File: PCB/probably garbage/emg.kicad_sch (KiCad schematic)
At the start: 102 parts, among them J1 USB_C_Receptacle_USB2.0_16P, J2 BAT+, J3 BAT-, SW1 RotaryEncoder_Switch_MP, SW10 2,2, SW11 2,3, SW12 2,4, SW13 2,5, SW14 3,1, SW15 3,2, SW16 3,3, SW17 3,4, SW18 3,5, SW19 4,1, SW2 EN, SW20 4,2, SW21 4,3, SW22 4,4, SW23 4,5, SW24 5,1, SW25 5,2, SW26 5,3, SW27 5,4, SW28 5,5, SW29 6,1, SW3 BOOT, SW30 6,2, SW31 6,3, SW32 6,4, SW33 6,5, SW34 7,1, SW35 7,2, SW36 7,3, SW37 7,4, SW38 7,5, SW4 1,1, SW5 1,2, SW6 1,3, SW7 1,4, SW8 1,5, SW9 2,1, U1 NCP1117-3.3_SOT223, U2 TVS1400DRV, U3 NCP1117-3.3_SOT223, U4 USBLC6-2SC6, U5 ESP32-C6-MINI-1

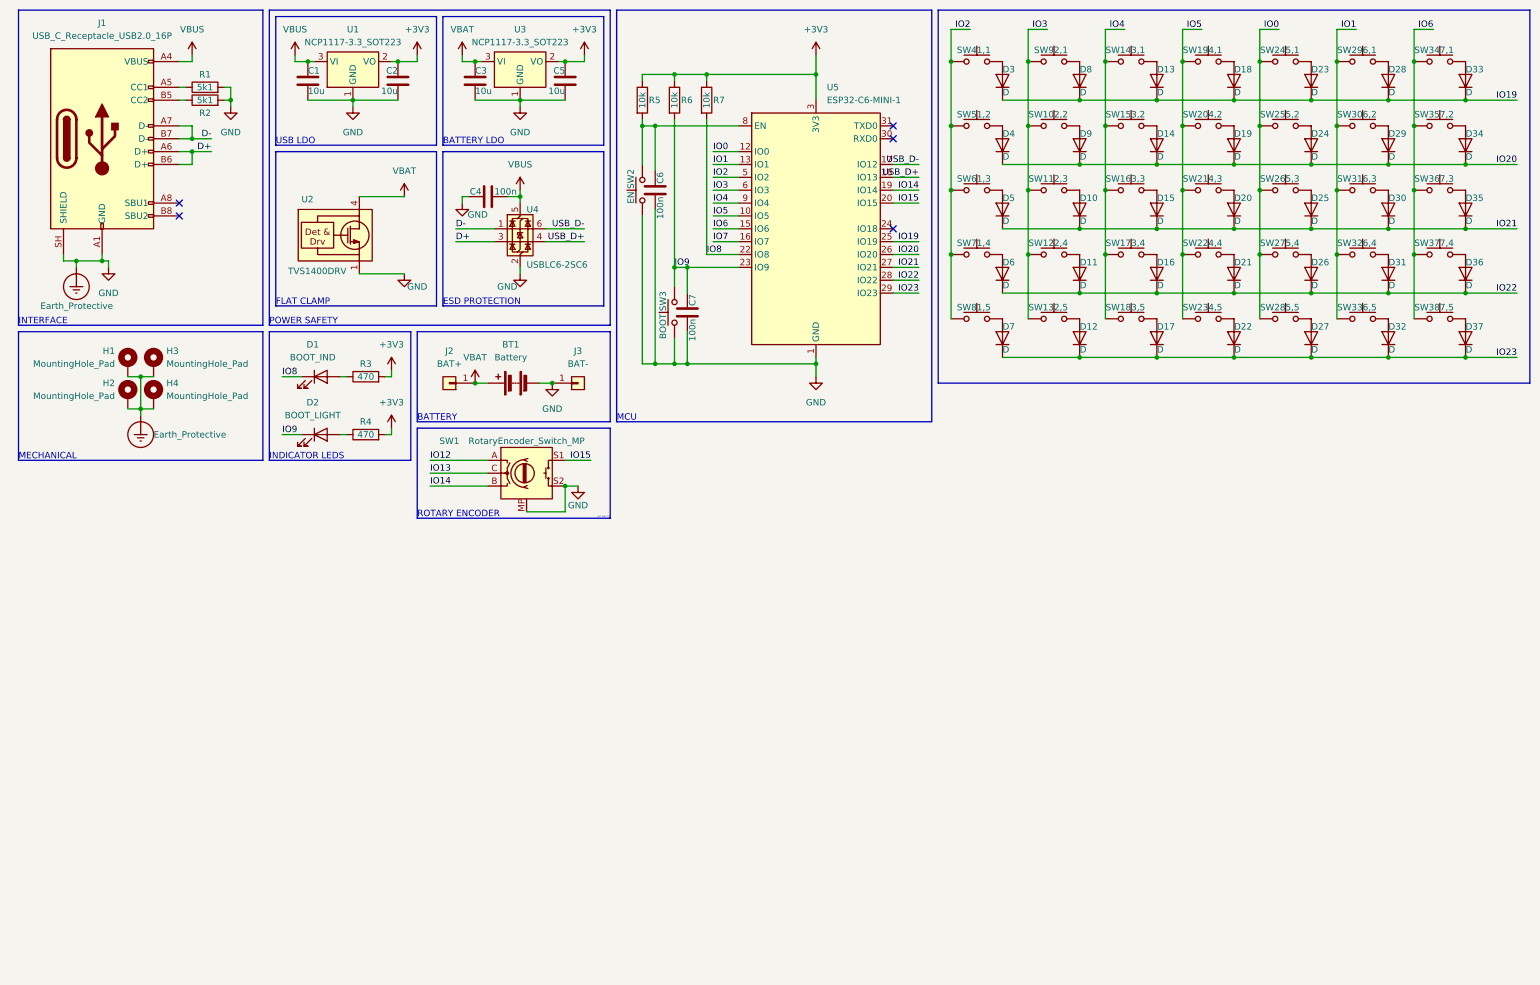
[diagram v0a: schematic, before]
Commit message: file organization
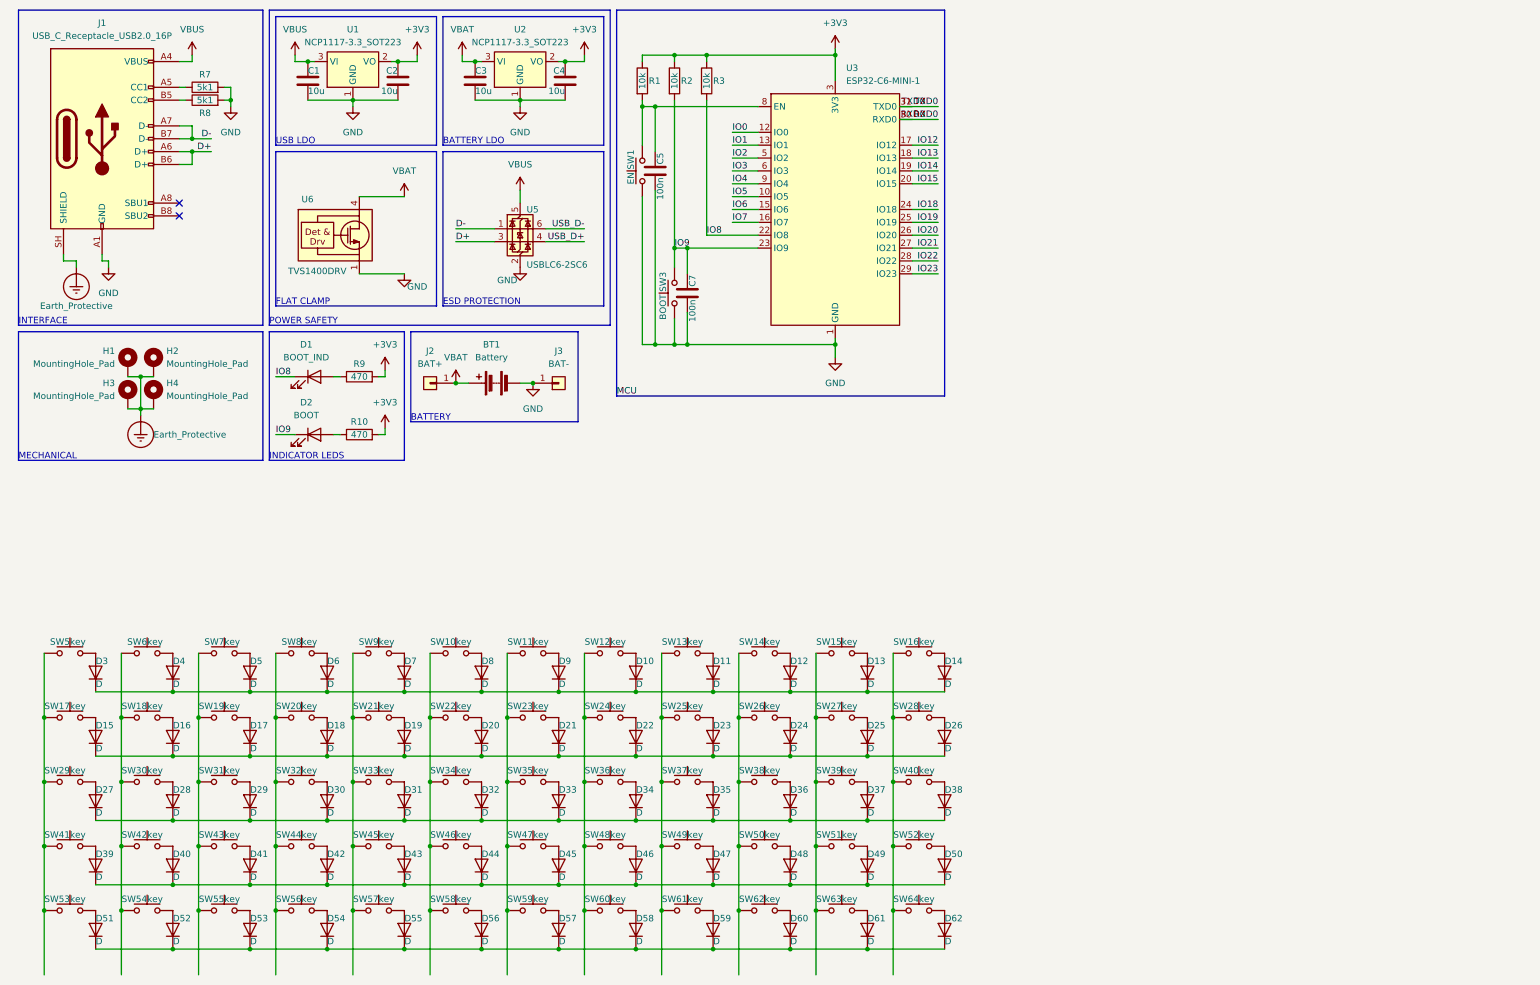
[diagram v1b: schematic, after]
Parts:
- removed C4: 100n, Diode_SMD:D_0805_2012Metric, symbol Device:C
- removed SW1: RotaryEncoder_Switch_MP, Rotary_Encoder:RotaryEncoder_Alps_EC12E-Switch_Vertical_H20mm_CircularMountingHoles, symbol Device:RotaryEncoder_Switch_MP
- added D10, D11, D12, D13, D14, D22, D23, D24, D25, D26, D34, D35, D36, D37, D38, D46, D47, D48, D49, D50, D58, D59, D60, D61, D62: D, symbol Device:D
- added SW12, SW13, SW14, SW15, SW16, SW24, SW25, SW26, SW27, SW28, SW36, SW37, SW38, SW39, SW40, SW48, SW49, SW50, SW51, SW52, SW60, SW61, SW62, SW63, SW64: key, symbol Switch:SW_Push
- BT1: footprint Battery:BatteryHolder_Keystone_1042_1x18650 -> (none)
- C1, C2, C3, C7, D1, D3: footprint Diode_SMD:D_0805_2012Metric -> (none)
- C4: renamed from C5; footprint Diode_SMD:D_0805_2012Metric -> (none)
- C5: renamed from C6; footprint Diode_SMD:D_0805_2012Metric -> (none)
- D15: renamed from D4; footprint Diode_SMD:D_0805_2012Metric -> (none)
- D16: renamed from D9; footprint Diode_SMD:D_0805_2012Metric -> (none)
- D17: renamed from D14; footprint Diode_SMD:D_0805_2012Metric -> (none)
- D18: renamed from D19; footprint Diode_SMD:D_0805_2012Metric -> (none)
- D19: renamed from D24; footprint Diode_SMD:D_0805_2012Metric -> (none)
- D2: value BOOT_LIGHT -> BOOT; footprint Diode_SMD:D_0805_2012Metric -> (none)
- D20: renamed from D29; footprint Diode_SMD:D_0805_2012Metric -> (none)
- D21: renamed from D34; footprint Diode_SMD:D_0805_2012Metric -> (none)
- D27: renamed from D5; footprint Diode_SMD:D_0805_2012Metric -> (none)
- D28: renamed from D10; footprint Diode_SMD:D_0805_2012Metric -> (none)
- D29: renamed from D15; footprint Diode_SMD:D_0805_2012Metric -> (none)
- D30: renamed from D20; footprint Diode_SMD:D_0805_2012Metric -> (none)
- D31: renamed from D25; footprint Diode_SMD:D_0805_2012Metric -> (none)
- D32: renamed from D30; footprint Diode_SMD:D_0805_2012Metric -> (none)
- D33: renamed from D35; footprint Diode_SMD:D_0805_2012Metric -> (none)
- D39: renamed from D6; footprint Diode_SMD:D_0805_2012Metric -> (none)
- D4: renamed from D8; footprint Diode_SMD:D_0805_2012Metric -> (none)
- D40: renamed from D11; footprint Diode_SMD:D_0805_2012Metric -> (none)
- D41: renamed from D16; footprint Diode_SMD:D_0805_2012Metric -> (none)
- D42: renamed from D21; footprint Diode_SMD:D_0805_2012Metric -> (none)
- D43: renamed from D26; footprint Diode_SMD:D_0805_2012Metric -> (none)
- D44: renamed from D31; footprint Diode_SMD:D_0805_2012Metric -> (none)
- D45: renamed from D36; footprint Diode_SMD:D_0805_2012Metric -> (none)
- D5: renamed from D13; footprint Diode_SMD:D_0805_2012Metric -> (none)
- D51: renamed from D7; footprint Diode_SMD:D_0805_2012Metric -> (none)
- D52: renamed from D12; footprint Diode_SMD:D_0805_2012Metric -> (none)
- D53: renamed from D17; footprint Diode_SMD:D_0805_2012Metric -> (none)
- D54: renamed from D22; footprint Diode_SMD:D_0805_2012Metric -> (none)
- D55: renamed from D27; footprint Diode_SMD:D_0805_2012Metric -> (none)
- D56: renamed from D32; footprint Diode_SMD:D_0805_2012Metric -> (none)
- D57: renamed from D37; footprint Diode_SMD:D_0805_2012Metric -> (none)
- D6: renamed from D18; footprint Diode_SMD:D_0805_2012Metric -> (none)
- D7: renamed from D23; footprint Diode_SMD:D_0805_2012Metric -> (none)
- D8: renamed from D28; footprint Diode_SMD:D_0805_2012Metric -> (none)
- D9: renamed from D33; footprint Diode_SMD:D_0805_2012Metric -> (none)
- H1, H4: footprint MountingHole:MountingHole_3.2mm_M3_Pad -> (none)
- H2: renamed from H3; footprint MountingHole:MountingHole_3.2mm_M3_Pad -> (none)
- H3: renamed from H2; footprint MountingHole:MountingHole_3.2mm_M3_Pad -> (none)
- J1: footprint Connector_USB:USB_C_Receptacle_GCT_USB4105-xx-A_16P_TopMnt_Horizontal -> (none)
- J2, J3: footprint Connector_PinHeader_2.54mm:PinHeader_1x01_P2.54mm_Vertical -> (none)
- R1: renamed from R5; footprint Capacitor_SMD:C_0603_1608Metric -> (none)
- R10: renamed from R4; footprint Capacitor_SMD:C_0603_1608Metric -> (none)
- R2: renamed from R6; footprint Capacitor_SMD:C_0603_1608Metric -> (none)
- R3: renamed from R7; footprint Capacitor_SMD:C_0603_1608Metric -> (none)
- R7: renamed from R1; footprint Capacitor_SMD:C_0603_1608Metric -> (none)
- R8: renamed from R2; footprint Capacitor_SMD:C_0603_1608Metric -> (none)
- R9: renamed from R3; footprint Capacitor_SMD:C_0603_1608Metric -> (none)
- SW1: renamed from SW2; footprint Button_Switch_SMD:SW_Push_SPST_NO_Alps_SKRK -> (none)
- SW10: renamed from SW29; value 6,1 -> key; footprint Button_Switch_Keyboard:SW_Cherry_MX_1.00u_PCB -> (none)
- SW11: renamed from SW34; value 7,1 -> key; footprint Button_Switch_Keyboard:SW_Cherry_MX_1.00u_PCB -> (none)
- SW17: renamed from SW5; value 1,2 -> key; footprint Button_Switch_Keyboard:SW_Cherry_MX_1.50u_PCB -> (none)
- SW18: renamed from SW10; value 2,2 -> key; footprint Button_Switch_Keyboard:SW_Cherry_MX_1.00u_PCB -> (none)
- SW19: renamed from SW15; value 3,2 -> key; footprint Button_Switch_Keyboard:SW_Cherry_MX_1.00u_PCB -> (none)
- SW20: value 4,2 -> key; footprint Button_Switch_Keyboard:SW_Cherry_MX_1.00u_PCB -> (none)
- SW21: renamed from SW25; value 5,2 -> key; footprint Button_Switch_Keyboard:SW_Cherry_MX_1.00u_PCB -> (none)
- SW22: renamed from SW30; value 6,2 -> key; footprint Button_Switch_Keyboard:SW_Cherry_MX_1.00u_PCB -> (none)
- SW23: renamed from SW35; value 7,2 -> key; footprint Button_Switch_Keyboard:SW_Cherry_MX_1.00u_PCB -> (none)
- SW29: renamed from SW6; value 1,3 -> key; footprint Button_Switch_Keyboard:SW_Cherry_MX_1.50u_PCB -> (none)
- SW3: footprint Button_Switch_SMD:SW_Push_SPST_NO_Alps_SKRK -> (none)
- SW30: renamed from SW11; value 2,3 -> key; footprint Button_Switch_Keyboard:SW_Cherry_MX_1.00u_PCB -> (none)
- SW31: renamed from SW16; value 3,3 -> key; footprint Button_Switch_Keyboard:SW_Cherry_MX_1.00u_PCB -> (none)
- SW32: renamed from SW21; value 4,3 -> key; footprint Button_Switch_Keyboard:SW_Cherry_MX_1.00u_PCB -> (none)
- SW33: renamed from SW26; value 5,3 -> key; footprint Button_Switch_Keyboard:SW_Cherry_MX_1.00u_PCB -> (none)
- SW34: renamed from SW31; value 6,3 -> key; footprint Button_Switch_Keyboard:SW_Cherry_MX_1.00u_PCB -> (none)
- SW35: renamed from SW36; value 7,3 -> key; footprint Button_Switch_Keyboard:SW_Cherry_MX_1.00u_PCB -> (none)
- SW41: renamed from SW7; value 1,4 -> key; footprint Button_Switch_Keyboard:SW_Cherry_MX_1.50u_PCB -> (none)
- SW42: renamed from SW12; value 2,4 -> key; footprint Button_Switch_Keyboard:SW_Cherry_MX_1.00u_PCB -> (none)
- SW43: renamed from SW17; value 3,4 -> key; footprint Button_Switch_Keyboard:SW_Cherry_MX_1.00u_PCB -> (none)
- SW44: renamed from SW22; value 4,4 -> key; footprint Button_Switch_Keyboard:SW_Cherry_MX_1.00u_PCB -> (none)
- SW45: renamed from SW27; value 5,4 -> key; footprint Button_Switch_Keyboard:SW_Cherry_MX_1.00u_PCB -> (none)
- SW46: renamed from SW32; value 6,4 -> key; footprint Button_Switch_Keyboard:SW_Cherry_MX_1.00u_PCB -> (none)
- SW47: renamed from SW37; value 7,4 -> key; footprint Button_Switch_Keyboard:SW_Cherry_MX_1.00u_PCB -> (none)
- SW5: renamed from SW4; value 1,1 -> key; footprint Button_Switch_Keyboard:SW_Cherry_MX_1.50u_PCB -> (none)
- SW53: renamed from SW8; value 1,5 -> key; footprint Button_Switch_Keyboard:SW_Cherry_MX_1.50u_PCB -> (none)
- SW54: renamed from SW13; value 2,5 -> key; footprint Button_Switch_Keyboard:SW_Cherry_MX_1.00u_PCB -> (none)
- SW55: renamed from SW18; value 3,5 -> key; footprint Button_Switch_Keyboard:SW_Cherry_MX_1.00u_PCB -> (none)
- SW56: renamed from SW23; value 4,5 -> key; footprint Button_Switch_Keyboard:SW_Cherry_MX_1.00u_PCB -> (none)
- SW57: renamed from SW28; value 5,5 -> key; footprint Button_Switch_Keyboard:SW_Cherry_MX_1.00u_PCB -> (none)
- SW58: renamed from SW33; value 6,5 -> key; footprint Button_Switch_Keyboard:SW_Cherry_MX_1.75u_PCB -> (none)
- SW59: renamed from SW38; value 7,5 -> key; footprint Button_Switch_Keyboard:SW_Cherry_MX_1.00u_PCB -> (none)
- SW6: renamed from SW9; value 2,1 -> key; footprint Button_Switch_Keyboard:SW_Cherry_MX_1.00u_PCB -> (none)
- SW7: renamed from SW14; value 3,1 -> key; footprint Button_Switch_Keyboard:SW_Cherry_MX_1.00u_PCB -> (none)
- SW8: renamed from SW19; value 4,1 -> key; footprint Button_Switch_Keyboard:SW_Cherry_MX_1.00u_PCB -> (none)
- SW9: renamed from SW24; value 5,1 -> key; footprint Button_Switch_Keyboard:SW_Cherry_MX_1.00u_PCB -> (none)
- renumbered U3 to U2, U5 to U3, U4 to U5, U2 to U6
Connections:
- net Earth_Protective: no longer BT1.2 (-), C1.2, C2.2, C3.2, C4.2, C5.2, C7.2, J1.A1 (GND), J1.A12 (GND), J1.B1 (GND), J1.B12 (GND), J3.1 (Pin_1), R7.2, R8.2, SW1.1, SW3.1, U1.1 (GND), U2.1 (GND), U3.1 (GND), U3.11 (GND), U3.14 (GND), U3.2 (GND), U3.36 (GND), U3.37 (GND), U3.38 (GND), U3.39 (GND), U3.40 (GND), U3.41 (GND), U3.42 (GND), U3.43 (GND), U3.44 (GND), U3.45 (GND), U3.46 (GND), U3.47 (GND), U3.48 (GND), U3.49 (GND), U3.50 (GND), U3.51 (GND), U3.52 (GND), U3.53 (GND), U5.2 (GND), U6.1 (GND), U6.2 (GND), U6.3 (GND), U6.7 (GND)
- net IO0: no longer SW21.1, SW33.1, SW45.1, SW57.1, SW9.1
- net IO1: no longer SW10.1, SW22.1, SW34.1, SW46.1, SW58.1
- net IO12: now also U3.17 (IO12)
- net IO13: now also U3.18 (IO13)
- net IO19: no longer D3.1 (K), D4.1 (K), D5.1 (K), D6.1 (K), D7.1 (K), D8.1 (K), D9.1 (K)
- net IO2: no longer SW17.1, SW29.1, SW41.1, SW5.1, SW53.1
- net IO20: no longer D15.1 (K), D16.1 (K), D17.1 (K), D18.1 (K), D19.1 (K), D20.1 (K), D21.1 (K)
- net IO21: no longer D27.1 (K), D28.1 (K), D29.1 (K), D30.1 (K), D31.1 (K), D32.1 (K), D33.1 (K)
- net IO22: no longer D39.1 (K), D40.1 (K), D41.1 (K), D42.1 (K), D43.1 (K), D44.1 (K), D45.1 (K)
- net IO23: no longer D51.1 (K), D52.1 (K), D53.1 (K), D54.1 (K), D55.1 (K), D56.1 (K), D57.1 (K)
- net IO3: no longer SW18.1, SW30.1, SW42.1, SW54.1, SW6.1
- net IO4: no longer SW19.1, SW31.1, SW43.1, SW55.1, SW7.1
- net IO5: no longer SW20.1, SW32.1, SW44.1, SW56.1, SW8.1
- net IO6: no longer SW11.1, SW23.1, SW35.1, SW47.1, SW59.1
- net USB_D+: no longer U3.18 (IO13)
- net USB_D-: no longer U3.17 (IO12)
- net IO18: now reaches U3.24 (IO18)
- new net: D39.1 (K), D40.1 (K), D41.1 (K), D42.1 (K), D43.1 (K), D44.1 (K), D45.1 (K), D46.1 (K), D47.1 (K), D48.1 (K), D49.1 (K), D50.1 (K)
- new net: D10.1 (K), D11.1 (K), D12.1 (K), D13.1 (K), D14.1 (K), D3.1 (K), D4.1 (K), D5.1 (K), D6.1 (K), D7.1 (K), D8.1 (K), D9.1 (K)
- new net: D51.1 (K), D52.1 (K), D53.1 (K), D54.1 (K), D55.1 (K), D56.1 (K), D57.1 (K), D58.1 (K), D59.1 (K), D60.1 (K), D61.1 (K), D62.1 (K)
- new net: D15.1 (K), D16.1 (K), D17.1 (K), D18.1 (K), D19.1 (K), D20.1 (K), D21.1 (K), D22.1 (K), D23.1 (K), D24.1 (K), D25.1 (K), D26.1 (K)
- new net: D25.2 (A), SW27.2
- new net: SW20.1, SW32.1, SW44.1, SW56.1, SW8.1
- new net: SW16.1, SW28.1, SW40.1, SW52.1, SW64.1
- new net: D26.2 (A), SW28.2
- new net: SW17.1, SW29.1, SW41.1, SW5.1, SW53.1
- new net: D27.1 (K), D28.1 (K), D29.1 (K), D30.1 (K), D31.1 (K), D32.1 (K), D33.1 (K), D34.1 (K), D35.1 (K), D36.1 (K), D37.1 (K), D38.1 (K)
- new net: D34.2 (A), SW36.2
- new net: SW13.1, SW25.1, SW37.1, SW49.1, SW61.1
- new net: D35.2 (A), SW37.2
- new net: SW10.1, SW22.1, SW34.1, SW46.1, SW58.1
- new net: SW21.1, SW33.1, SW45.1, SW57.1, SW9.1
- new net: D12.2 (A), SW14.2
- new net: D14.2 (A), SW16.2
- new net: SW12.1, SW24.1, SW36.1, SW48.1, SW60.1
- new net: D46.2 (A), SW48.2
- new net: SW11.1, SW23.1, SW35.1, SW47.1, SW59.1
- new net: D50.2 (A), SW52.2
- new net: D49.2 (A), SW51.2
- new net: SW19.1, SW31.1, SW43.1, SW55.1, SW7.1
- new net: D10.2 (A), SW12.2
- new net: D22.2 (A), SW24.2
- new net: SW18.1, SW30.1, SW42.1, SW54.1, SW6.1
- new net: D61.2 (A), SW63.2
- new net: D36.2 (A), SW38.2
- new net: SW15.1, SW27.1, SW39.1, SW51.1, SW63.1
- new net: D37.2 (A), SW39.2
- new net: D60.2 (A), SW62.2
- new net: D13.2 (A), SW15.2
- new net: D24.2 (A), SW26.2
- new net: D23.2 (A), SW25.2
- new net: SW14.1, SW26.1, SW38.1, SW50.1, SW62.1
- new net: D59.2 (A), SW61.2
- new net: D47.2 (A), SW49.2
- new net: D48.2 (A), SW50.2
- new net: D62.2 (A), SW64.2
- new net: D58.2 (A), SW60.2
- new net: D11.2 (A), SW13.2
- new net: D38.2 (A), SW40.2
- new net GND: BT1.2 (-), C1.2, C2.2, C3.2, C4.2, C5.2, C7.2, J1.A1 (GND), J1.A12 (GND), J1.B1 (GND), J1.B12 (GND), J3.1 (Pin_1), R7.2, R8.2, SW1.1, SW3.1, U1.1 (GND), U2.1 (GND), U3.1 (GND), U3.11 (GND), U3.14 (GND), U3.2 (GND), U3.36 (GND), U3.37 (GND), U3.38 (GND), U3.39 (GND), U3.40 (GND), U3.41 (GND), U3.42 (GND), U3.43 (GND), U3.44 (GND), U3.45 (GND), U3.46 (GND), U3.47 (GND), U3.48 (GND), U3.49 (GND), U3.50 (GND), U3.51 (GND), U3.52 (GND), U3.53 (GND), U5.2 (GND), U6.1 (GND), U6.2 (GND), U6.3 (GND), U6.7 (GND)
- no-connect marks 5 -> 2
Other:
- note removed: "(nah really???)"
- note removed: "MCU"
- note removed: "ROTARY ENCODER"
- moved on the sheet: BT1, C5, C7, D1, D15, D16, D17, D18, D19, D2, D20, D21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
